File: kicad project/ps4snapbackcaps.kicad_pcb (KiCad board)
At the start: 2 copper layers, 14 x 15.2 mm, 4 parts

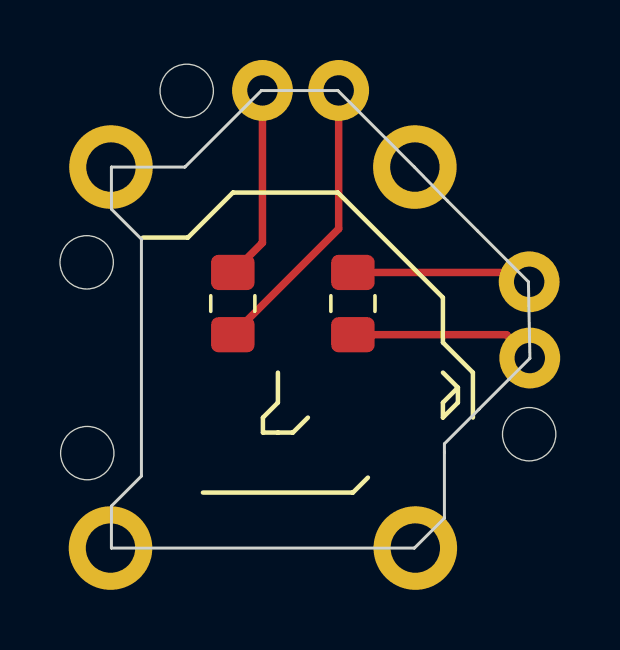
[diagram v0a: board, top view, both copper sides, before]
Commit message: oopsie!
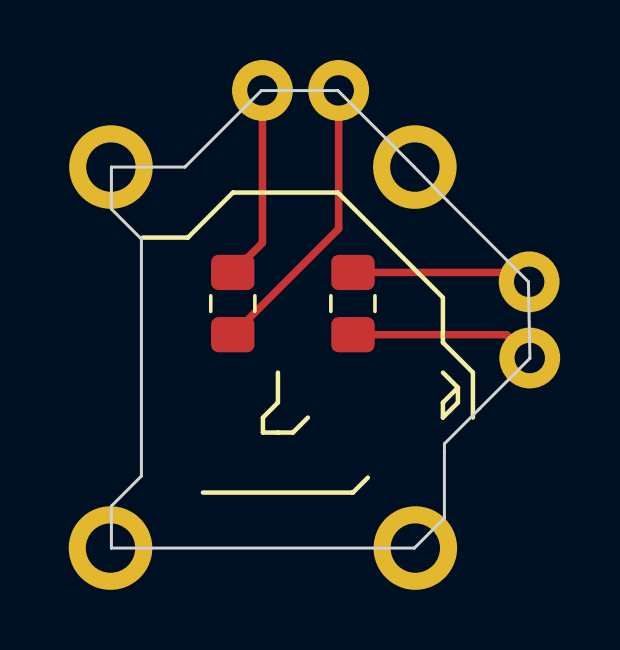
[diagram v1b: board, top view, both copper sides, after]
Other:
- board text added: "sable's DualShock 4 Snapback Capacitor Board V1.1"
- board text removed: "Stevano's DualShock 4 Snapback Capacitor Board V1.0"
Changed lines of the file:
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@@
       (usegerberattributes true)
       (usegerberadvancedattributes true)
-      (creategerberjobfile true)
+      (creategerberjobfile false)
       (dashed_line_dash_ratio 12.000000)
       (dashed_line_gap_ratio 3.000000)
@@
       (outputformat 1)
       (mirror false)
-      (drillshape 1)
+      (drillshape 0)
       (scaleselection 1)
-      (outputdirectory "")
+      (outputdirectory "C:/Users/steve/Downloads/gerbers/")
     )
   )
@@
     (fp_line (start 1 0.625) (end -1 0.625)
       (stroke (width 0.1) (type solid)) (layer "F.Fab"))
-    (pad "1" smd roundrect (at -1.0375 0 270) (size 1.175 1.45) (layers "F.Cu" "F.Paste" "F.Mask") (roundrect_rratio 0.212766)
+    (pad "1" smd roundrect (at -1.0375 0 270) (size 1.175 1.45) (layers "F.Cu" "F.Paste" "F.Mask") (roundrect_rratio 0.2127659574)
       (net 1 "Net-(U1-V)") (pintype "passive"))
-    (pad "2" smd roundrect (at 1.0375 0 270) (size 1.175 1.45) (layers "F.Cu" "F.Paste" "F.Mask") (roundrect_rratio 0.212766)
+    (pad "2" smd roundrect (at 1.0375 0 270) (size 1.175 1.45) (layers "F.Cu" "F.Paste" "F.Mask") (roundrect_rratio 0.2127659574)
       (net 2 "Net-(U1-V-)") (pintype "passive"))
-    (model "${KICAD6_3DMODEL_DIR}/Capacitor_SMD.3dshapes/C_0805_2012Metric.wrl"
+    (model "${KICAD7_3DMODEL_DIR}/Capacitor_SMD.3dshapes/C_0805_2012Metric.wrl"
       (offset (xyz 0 0 0))
       (scale (xyz 1 1 1))
@@
     (fp_line (start 1 0.625) (end -1 0.625)
       (stroke (width 0.1) (type solid)) (layer "F.Fab"))
-    (pad "1" smd roundrect (at -1.0375 0 90) (size 1.175 1.45) (layers "F.Cu" "F.Paste" "F.Mask") (roundrect_rratio 0.212766)
+    (pad "1" smd roundrect (at -1.0375 0 90) (size 1.175 1.45) (layers "F.Cu" "F.Paste" "F.Mask") (roundrect_rratio 0.2127659574)
       (net 3 "Net-(U1-H)") (pintype "passive"))
-    (pad "2" smd roundrect (at 1.0375 0 90) (size 1.175 1.45) (layers "F.Cu" "F.Paste" "F.Mask") (roundrect_rratio 0.212766)
+    (pad "2" smd roundrect (at 1.0375 0 90) (size 1.175 1.45) (layers "F.Cu" "F.Paste" "F.Mask") (roundrect_rratio 0.2127659574)
       (net 4 "Net-(U1-H-)") (pintype "passive"))
-    (model "${KICAD6_3DMODEL_DIR}/Capacitor_SMD.3dshapes/C_0805_2012Metric.wrl"
+    (model "${KICAD7_3DMODEL_DIR}/Capacitor_SMD.3dshapes/C_0805_2012Metric.wrl"
       (offset (xyz 0 0 0))
       (scale (xyz 1 1 1))
@@
         (effects (font (size 1 1) (thickness 0.15)) (justify mirror))
     )
-    (pad "" np_thru_hole circle (at -8.89 2.54 270) (size 1.778 1.778) (drill 1.778) (layers "F&B.Cu" "*.Mask"))
-    (pad "" np_thru_hole circle (at -3.175 5.8748 270) (size 1.778 1.778) (drill 1.778) (layers "F&B.Cu" "*.Mask"))
-    (pad "" np_thru_hole circle (at 2.555 -8.8752 270) (size 1.778 1.778) (drill 1.778) (layers "F&B.Cu" "*.Mask"))
-    (pad "" np_thru_hole circle (at 3.185 5.8548 270) (size 1.778 1.778) (drill 1.778) (layers "F&B.Cu" "*.Mask"))
     (pad "H2" thru_hole circle (at 0.015 -8.8952 270) (size 2.028 2.028) (drill 1.014) (property pad_prop_castellated) (layers "*.Cu" "*.Mask")
       (net 3 "Net-(U1-H)") (pinfunction "H") (pintype "output"))
@@
     (effects (font (size 0.8 0.8) (thickness 0.15)) (justify left bottom mirror))
   )
-  (gr_text "Stevano's\nDualShock 4\nSnapback\nCapacitor\nBoard V1.0" (at 86 72.5) (layer "B.SilkS")
+  (gr_text "sable's\nDualShock 4\nSnapback\nCapacitor\nBoard V1.1" (at 86 72.5) (layer "B.SilkS")
     (effects (font (size 0.8 0.8) (thickness 0.15)) (justify mirror))
   )
@@
   (segment (start 88 71.1625) (end 93.360724 71.1625) (width 0.25) (layer "F.Cu") (net 4))
   (segment (start 93.360724 71.1625) (end 93.673224 71.475) (width 0.25) (layer "F.Cu") (net 4))
-  (group "" (id cb654c15-b03d-4eb5-844a-dd08d4b6b979)
-    (members
-      7a339b87-1b18-4104-ba1b-928e2e3e2476
-      cb7d4074-78d4-4b05-bf72-795e81b908d6
-    )
-  )
 )
